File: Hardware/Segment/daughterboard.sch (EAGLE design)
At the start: 175 parts, among them IC1 PBQ79656PAPTQ1, IC2 PBQ79656PAPTQ1, T1 PBHV8115X, 115, T2 PBHV8115X, 115

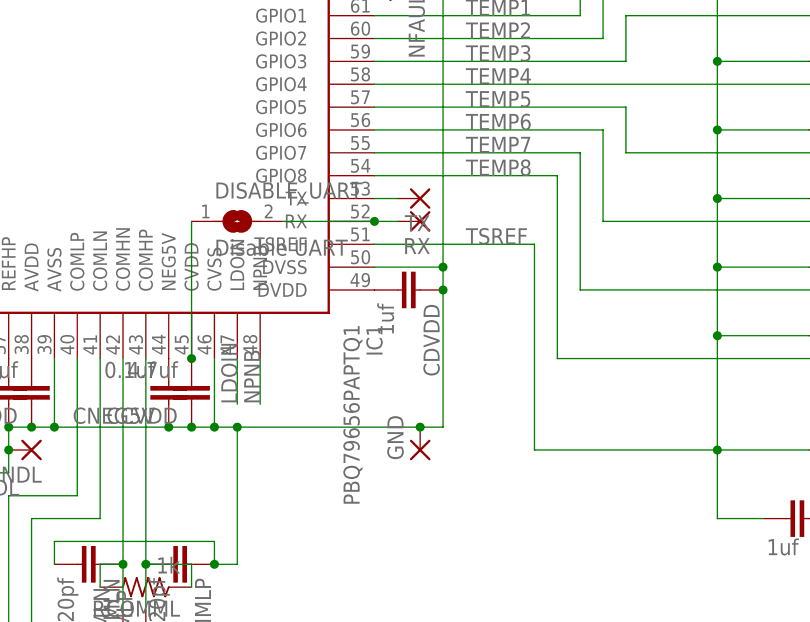
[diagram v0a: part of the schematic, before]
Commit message: Daughterboard fixes V2.1
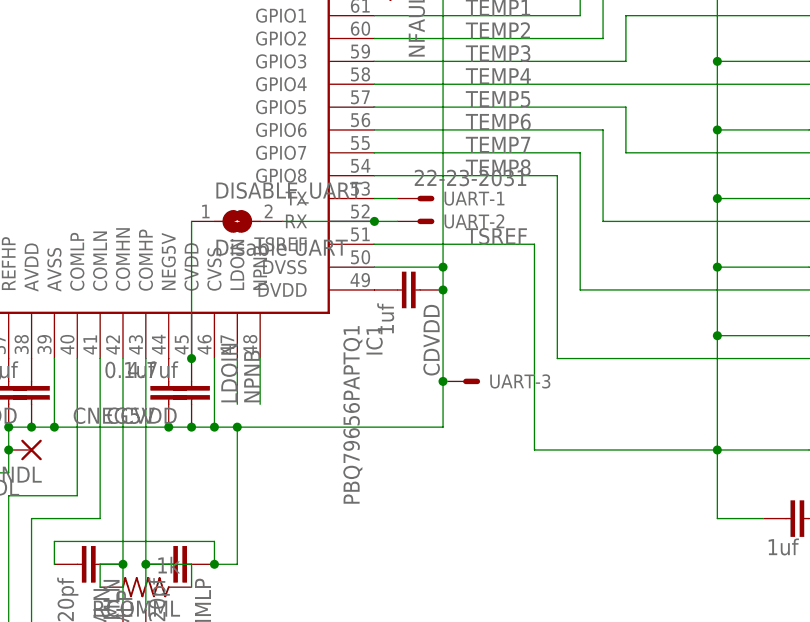
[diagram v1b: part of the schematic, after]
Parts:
- removed GND, RX, TX: (no value), wirepad:2,54/1,0
- added UART: 22-23-2031, con-molex:22-23-2031
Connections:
- net GNDL: now also UART-3.S; no longer GND.P
- net N$3: now also UART-2.S; no longer RX.P
- net N$9: now also UART-1.S; no longer TX.P
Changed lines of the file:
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@@
 <part name="GNDL" library="wirepad" library_urn="urn:adsk.eagle:library:412" deviceset="SMD5" device="" package3d_urn="urn:adsk.eagle:package:30841/1"/>
 <part name="GNDH" library="wirepad" library_urn="urn:adsk.eagle:library:412" deviceset="SMD5" device="" package3d_urn="urn:adsk.eagle:package:30841/1"/>
-<part name="TX" library="wirepad" library_urn="urn:adsk.eagle:library:412" deviceset="2,54/1,0" device="" package3d_urn="urn:adsk.eagle:package:30828/1"/>
-<part name="RX" library="wirepad" library_urn="urn:adsk.eagle:library:412" deviceset="2,54/1,0" device="" package3d_urn="urn:adsk.eagle:package:30828/1"/>
-<part name="GND" library="wirepad" library_urn="urn:adsk.eagle:library:412" deviceset="2,54/1,0" device="" package3d_urn="urn:adsk.eagle:package:30828/1"/>
 <part name="NFAULT" library="testpad" library_urn="urn:adsk.eagle:library:385" deviceset="TP" device="B2,54" package3d_urn="urn:adsk.eagle:package:27948/1"/>
 <part name="RCS1" library="rcl" library_urn="urn:adsk.eagle:library:334" deviceset="R-US_" device="R0603" package3d_urn="urn:adsk.eagle:package:23555/3" value="10"/>
@@
 <part name="CCB10" library="rcl" library_urn="urn:adsk.eagle:library:334" deviceset="C-EU" device="C0603" package3d_urn="urn:adsk.eagle:package:23616/2" value="0.47uf"/>
 <part name="CCB10-1" library="rcl" library_urn="urn:adsk.eagle:library:334" deviceset="C-EU" device="C0603" package3d_urn="urn:adsk.eagle:package:23616/2" value="0.47uf"/>
+<part name="UART" library="con-molex" library_urn="urn:adsk.eagle:library:165" deviceset="22-23-2031" device="" package3d_urn="urn:adsk.eagle:package:8078634/1"/>
 </parts>
 <sheets>
@@
 <attribute name="VALUE" x="145.923" y="270.002" size="1.778" layer="96" rot="R180"/>
 </instance>
-<instance part="TX" gate="P" x="195.58" y="45.72" smashed="yes" rot="R180">
-<attribute name="NAME" x="196.723" y="43.8658" size="1.778" layer="95" rot="R180"/>
-<attribute name="VALUE" x="196.723" y="49.022" size="1.778" layer="96" rot="R180"/>
-</instance>
-<instance part="RX" gate="P" x="195.58" y="43.18" smashed="yes" rot="R180">
-<attribute name="NAME" x="196.723" y="41.3258" size="1.778" layer="95" rot="R180"/>
-<attribute name="VALUE" x="196.723" y="46.482" size="1.778" layer="96" rot="R180"/>
-</instance>
-<instance part="GND" gate="P" x="195.58" y="17.78" smashed="yes" rot="R90">
-<attribute name="NAME" x="193.7258" y="16.637" size="1.778" layer="95" rot="R90"/>
-<attribute name="VALUE" x="198.882" y="16.637" size="1.778" layer="96" rot="R90"/>
-</instance>
 <instance part="NFAULT" gate="G$1" x="193.04" y="68.58" smashed="yes" rot="R270">
 <attribute name="NAME" x="194.31" y="69.85" size="1.778" layer="95" rot="R270"/>
@@
 <attribute name="NAME" x="136.779" y="339.344" size="1.778" layer="95" rot="R90"/>
 <attribute name="VALUE" x="141.859" y="339.344" size="1.778" layer="96" rot="R90"/>
+</instance>
+<instance part="UART" gate="-1" x="195.58" y="45.72" smashed="yes">
+<attribute name="NAME" x="198.12" y="44.958" size="1.524" layer="95"/>
+<attribute name="VALUE" x="194.818" y="47.117" size="1.778" layer="96"/>
+</instance>
+<instance part="UART" gate="-2" x="195.58" y="43.18" smashed="yes">
+<attribute name="NAME" x="198.12" y="42.418" size="1.524" layer="95"/>
+</instance>
+<instance part="UART" gate="-3" x="200.66" y="25.4" smashed="yes">
+<attribute name="NAME" x="203.2" y="24.638" size="1.524" layer="95"/>
 </instance>
 </instances>
@@
 <pinref part="CDVDD" gate="G$1" pin="1"/>
 <wire x1="198.12" y1="38.1" x2="198.12" y2="35.56" width="0.1524" layer="91"/>
-<wire x1="198.12" y1="35.56" x2="198.12" y2="20.32" width="0.1524" layer="91"/>
-<wire x1="198.12" y1="20.32" x2="195.58" y2="20.32" width="0.1524" layer="91"/>
+<wire x1="198.12" y1="35.56" x2="198.12" y2="25.4" width="0.1524" layer="91"/>
 <junction x="198.12" y="35.56"/>
 <junction x="172.72" y="20.32"/>
 <pinref part="IC1" gate="G$1" pin="AVSS?"/>
-<wire x1="195.58" y1="20.32" x2="175.26" y2="20.32" width="0.1524" layer="91"/>
+<wire x1="198.12" y1="25.4" x2="198.12" y2="20.32" width="0.1524" layer="91"/>
+<wire x1="198.12" y1="20.32" x2="175.26" y2="20.32" width="0.1524" layer="91"/>
 <wire x1="175.26" y1="20.32" x2="172.72" y2="20.32" width="0.1524" layer="91"/>
 <wire x1="190.5" y1="76.2" x2="198.12" y2="76.2" width="0.1524" layer="91"/>
@@
 <pinref part="GNDL" gate="1" pin="P"/>
 <junction x="149.86" y="17.78"/>
-<pinref part="GND" gate="P" pin="P"/>
-<junction x="195.58" y="20.32"/>
+<pinref part="UART" gate="-3" pin="S"/>
+<junction x="198.12" y="25.4"/>
 </segment>
 <segment>
@@
 <wire x1="180.34" y1="43.18" x2="190.5" y2="43.18" width="0.1524" layer="91"/>
 <wire x1="193.04" y1="43.18" x2="190.5" y2="43.18" width="0.1524" layer="91"/>
-<pinref part="RX" gate="P" pin="P"/>
 <junction x="190.5" y="43.18"/>
+<pinref part="UART" gate="-2" pin="S"/>
 </segment>
 </net>
@@
 <pinref part="IC1" gate="G$1" pin="TX"/>
 <wire x1="193.04" y1="45.72" x2="190.5" y2="45.72" width="0.1524" layer="91"/>
-<pinref part="TX" gate="P" pin="P"/>
-</segment>
-</net>
+<pinref part="UART" gate="-1" pin="S"/>
+</segment>
+</net>
